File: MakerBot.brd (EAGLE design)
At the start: 152.7 x 118.7 mm, 52 parts, among them U10 MCP4018, U11 MCP4018, U8 MCP4018, U9 MCP4018

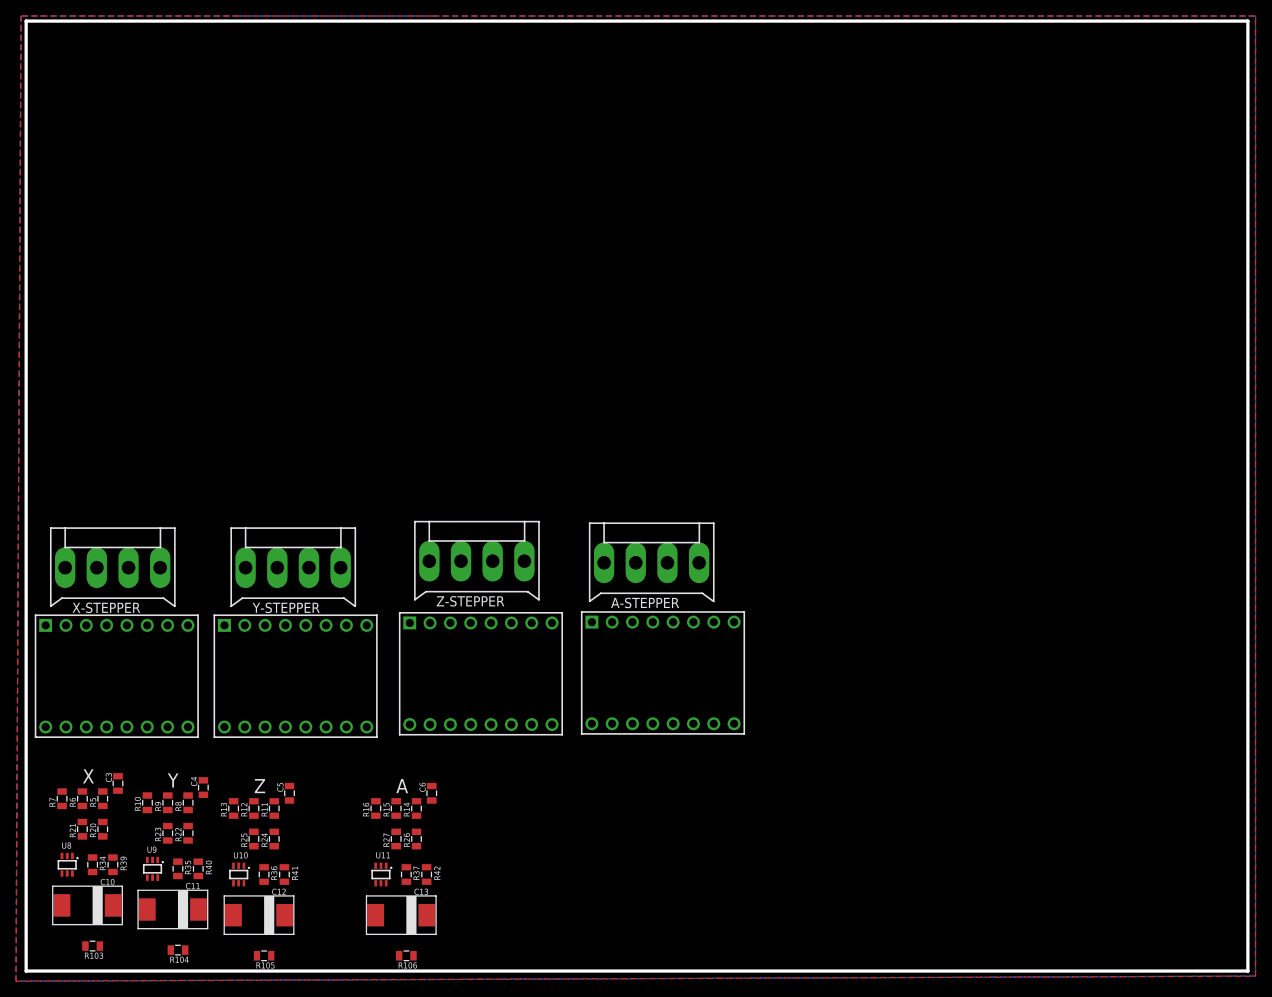
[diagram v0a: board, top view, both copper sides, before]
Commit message: Designed! Routed! Time to build!
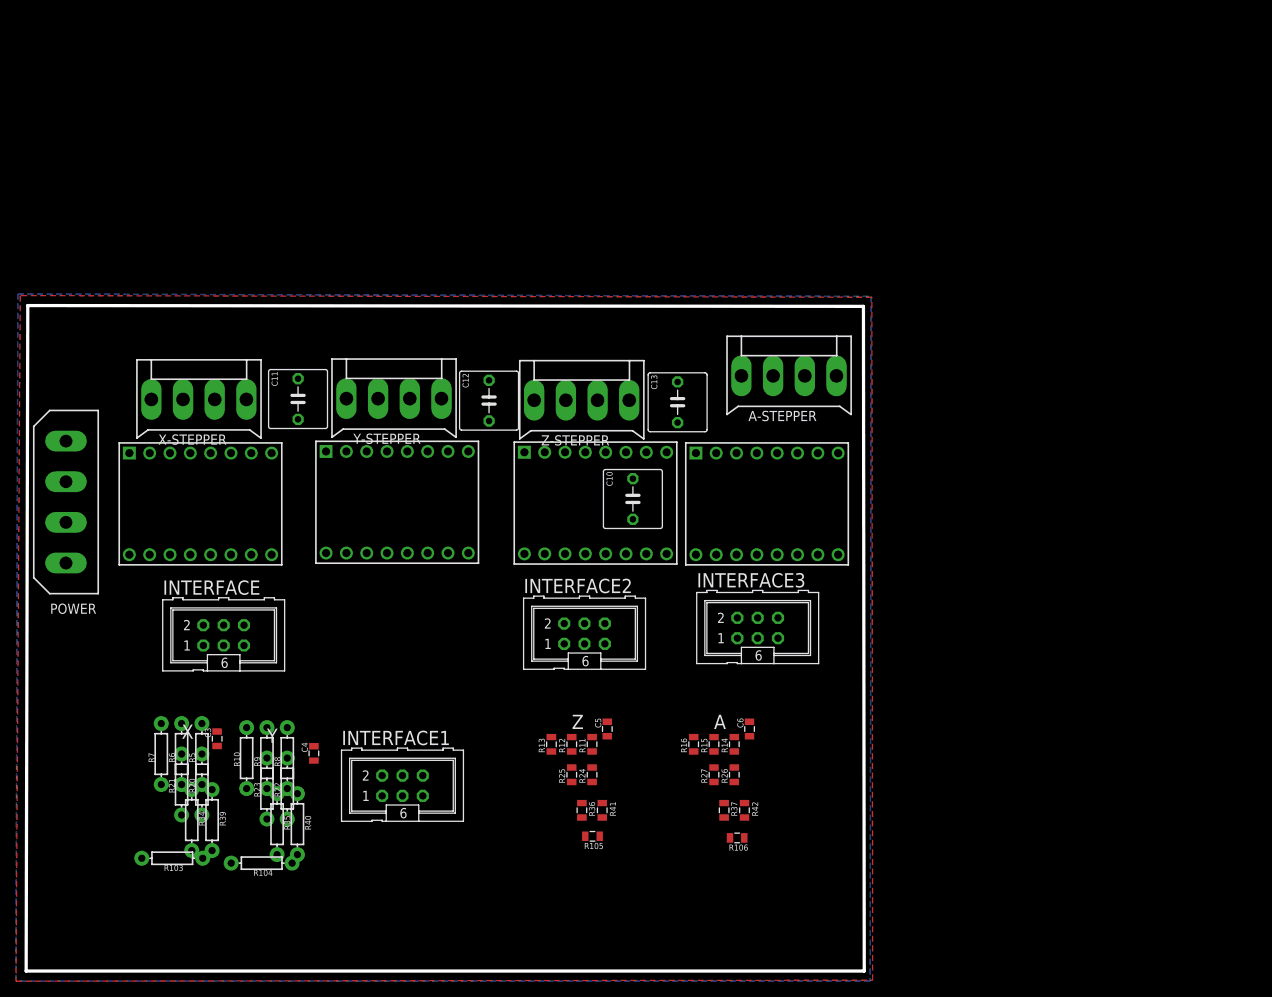
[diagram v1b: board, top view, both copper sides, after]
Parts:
- removed U10, U11, U8, U9: MCP4018, MakerBot:SC70-6L
- added INTERFACE, INTERFACE1, INTERFACE2, INTERFACE3: (no value), con-ml:ML6
- added POWER: 9090-4V, con-thomas-betts:9090-4V
- C10, C11, C12, C13: device adafruit:CAP2917 -> adafruit:C050-075X075
- R10, R103, R104, R20, R21, R22, R23, R34, R35, R39, R40, R5, R6, R7, R8, R9: device SparkFun:0805 -> SparkFun:AXIAL-0.3
- moved C10 85.0 mm to (75.8, 59.0), turned to 270 degrees
- moved C13 72.8 mm to (81.4, 71.1), turned to 270 degrees
- moved C12 70.4 mm to (57.9, 71.3), turned to 270 degrees
- moved C11 65.7 mm to (34.0, 71.5), turned to 270 degrees
- moved R106 43.9 mm to (88.9, 16.6)
- moved R105 43.7 mm to (70.8, 16.8)
- moved C5 40.5 mm to (72.6, 30.3)
- moved C6 40.5 mm to (90.4, 30.3)
- moved R13 40.5 mm to (65.7, 28.3)
- moved R14 40.5 mm to (88.5, 28.3)
- moved R26 40.5 mm to (88.5, 24.5)
- moved R11 40.5 mm to (70.7, 28.3)
- moved R12 40.5 mm to (68.2, 28.3)
- moved R15 40.5 mm to (86.0, 28.3)
- moved R24 40.5 mm to (70.7, 24.5)
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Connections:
- removed net A-AXIS-POT: R106.2
- removed net N$112: R35.1, U9.6
- removed net N$126: R36.1, U10.6
- removed net N$176: R37.1, U11.6
- removed net N$356: R103.1, U8.4
- removed net N$357: R104.1, U9.4
- removed net N$359: R105.1, U10.4
- removed net N$361: R106.1, U11.4
- removed net N$98: R34.1, U8.6
- removed net POTS-SCL: U10.3, U11.3, U8.3, U9.3
- removed net X-AXIS-POT: R103.2
- removed net Y-AXIS-POT: R104.2
- removed net Z-AXIS-POT: R105.2
- new net N$1: R15.1, R27.2
- new net N$2: R14.1, R26.2
- new net RESET: INTERFACE.6, INTERFACE1.6, INTERFACE2.6, INTERFACE3.6
- net +24V: now also POWER.4
- net 5V: now also POWER.1, R10.P$2, R34.P$2, R35.P$2, R39.P$2, R40.P$2, R5.P$2, R6.P$2, R7.P$2, R8.P$2, R9.P$2; no longer R10.2, R34.2, R35.2, R39.2, R40.2, R5.2, R6.2, R7.2, R8.2, R9.2, U10.1, U11.1, U8.1, U9.1
- net A-AXIS-DIR: now also INTERFACE3.4
- net A-AXIS-EN: now also INTERFACE3.5
- net A-AXIS-STEP: now also INTERFACE3.3
- net GND: now also INTERFACE.1, INTERFACE.2, INTERFACE1.1, INTERFACE1.2, INTERFACE2.1, INTERFACE2.2, INTERFACE3.1, INTERFACE3.2, POWER.2, POWER.3, R20.P$1, R21.P$1, R22.P$1, R23.P$1; no longer R20.1, R21.1, R22.1, R23.1, U10.2, U11.2, U8.2, U9.2
- net N$100: now also R21.P$2, R6.P$1; no longer R21.2, R6.1
- net N$102: now also R10.P$1; no longer R10.1
- net N$111: no longer U9.5
- net N$114: now also R23.P$2, R9.P$1; no longer R23.2, R9.1
- net N$121: now also R22.P$2, R8.P$1; no longer R22.2, R8.1
- net N$124: no longer U10.5
- net N$173: no longer U11.5
- net N$177: no longer R15.1, R27.2
- net N$18: now also R20.P$2, R5.P$1; no longer R20.2, R5.1
- net N$188: no longer R14.1, R26.2
- net N$37: now also R7.P$1; no longer R7.1
- net N$96: no longer U8.5
- net X-AXIS-DIR: now also INTERFACE.4
- net X-AXIS-EN: now also INTERFACE.5, R39.P$1; no longer R39.1
- net X-AXIS-STEP: now also INTERFACE.3
- net Y-AXIS-DIR: now also INTERFACE1.4
- net Y-AXIS-EN: now also INTERFACE1.5, R40.P$1; no longer R40.1
- net Y-AXIS-STEP: now also INTERFACE1.3
- net Z-AXIS-DIR: now also INTERFACE2.4
- net Z-AXIS-EN: now also INTERFACE2.5
- net Z-AXIS-STEP: now also INTERFACE2.3
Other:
- board size 152.7 x 118.7 mm -> 104.8 x 83.2 mm
